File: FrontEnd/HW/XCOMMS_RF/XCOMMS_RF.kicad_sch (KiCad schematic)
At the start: 54 parts, among them J1 SMA, J2 SMA, J3 SFC-110-T2-F-D-A-TR, U1 SIM-14+, U2 HMC788ALP2ETR, U3 HMC952ALP5GE, U5 HMC788ALP2ETR, U6 AD8031, U7 ADT7310

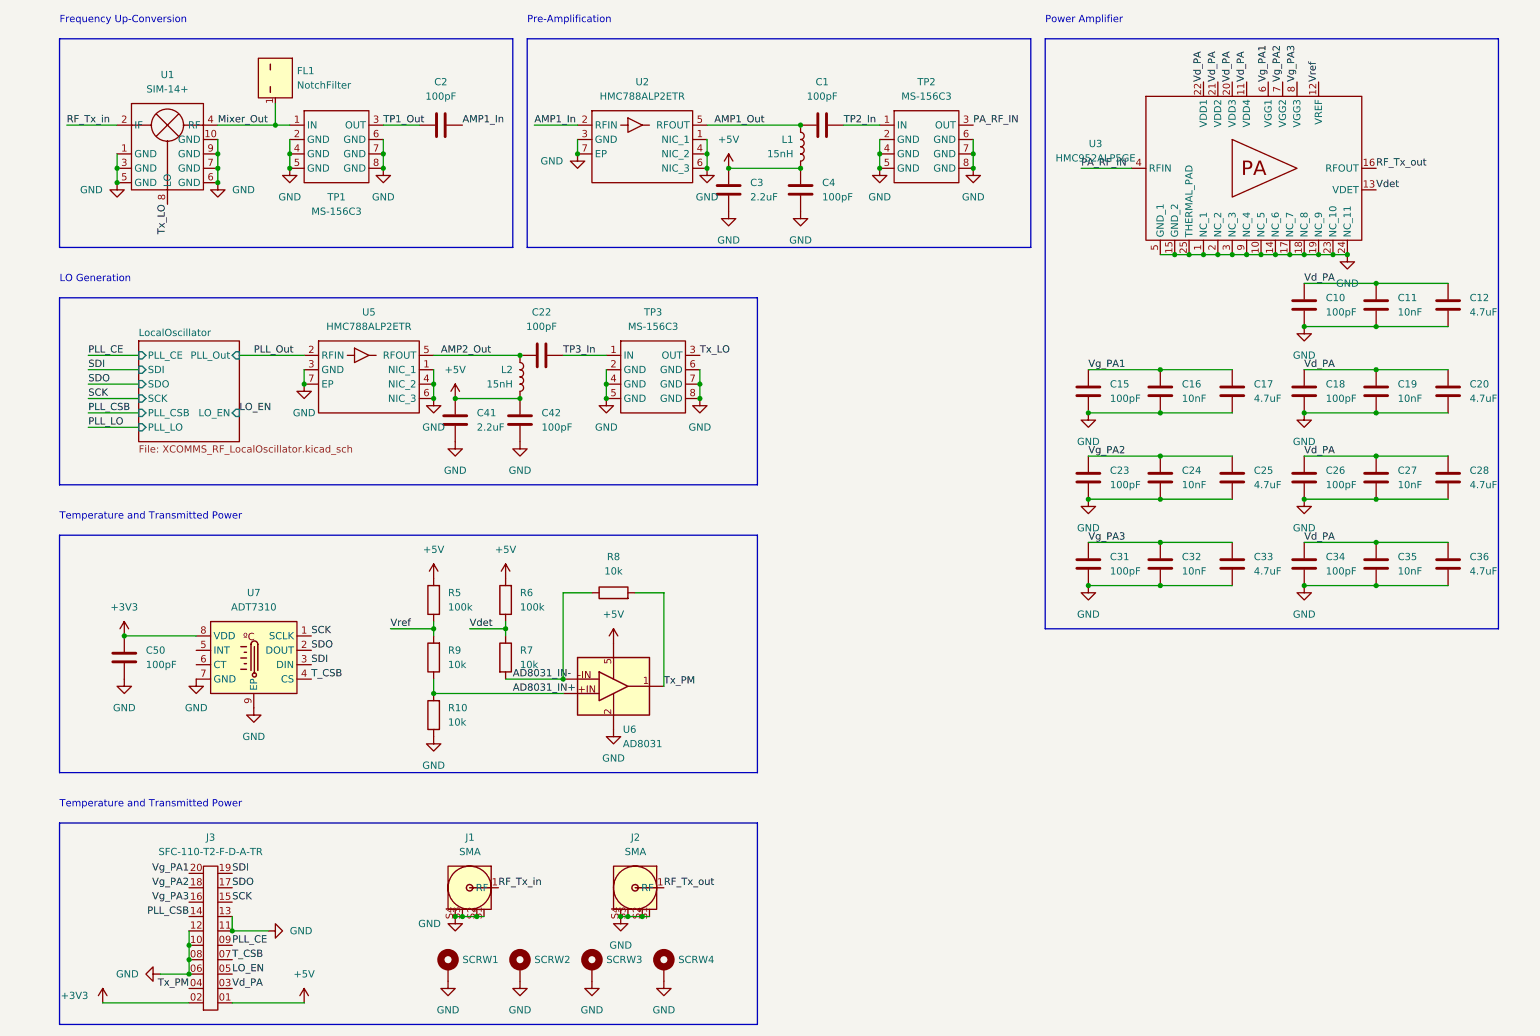
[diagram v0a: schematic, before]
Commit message: XCOMMS_RF update
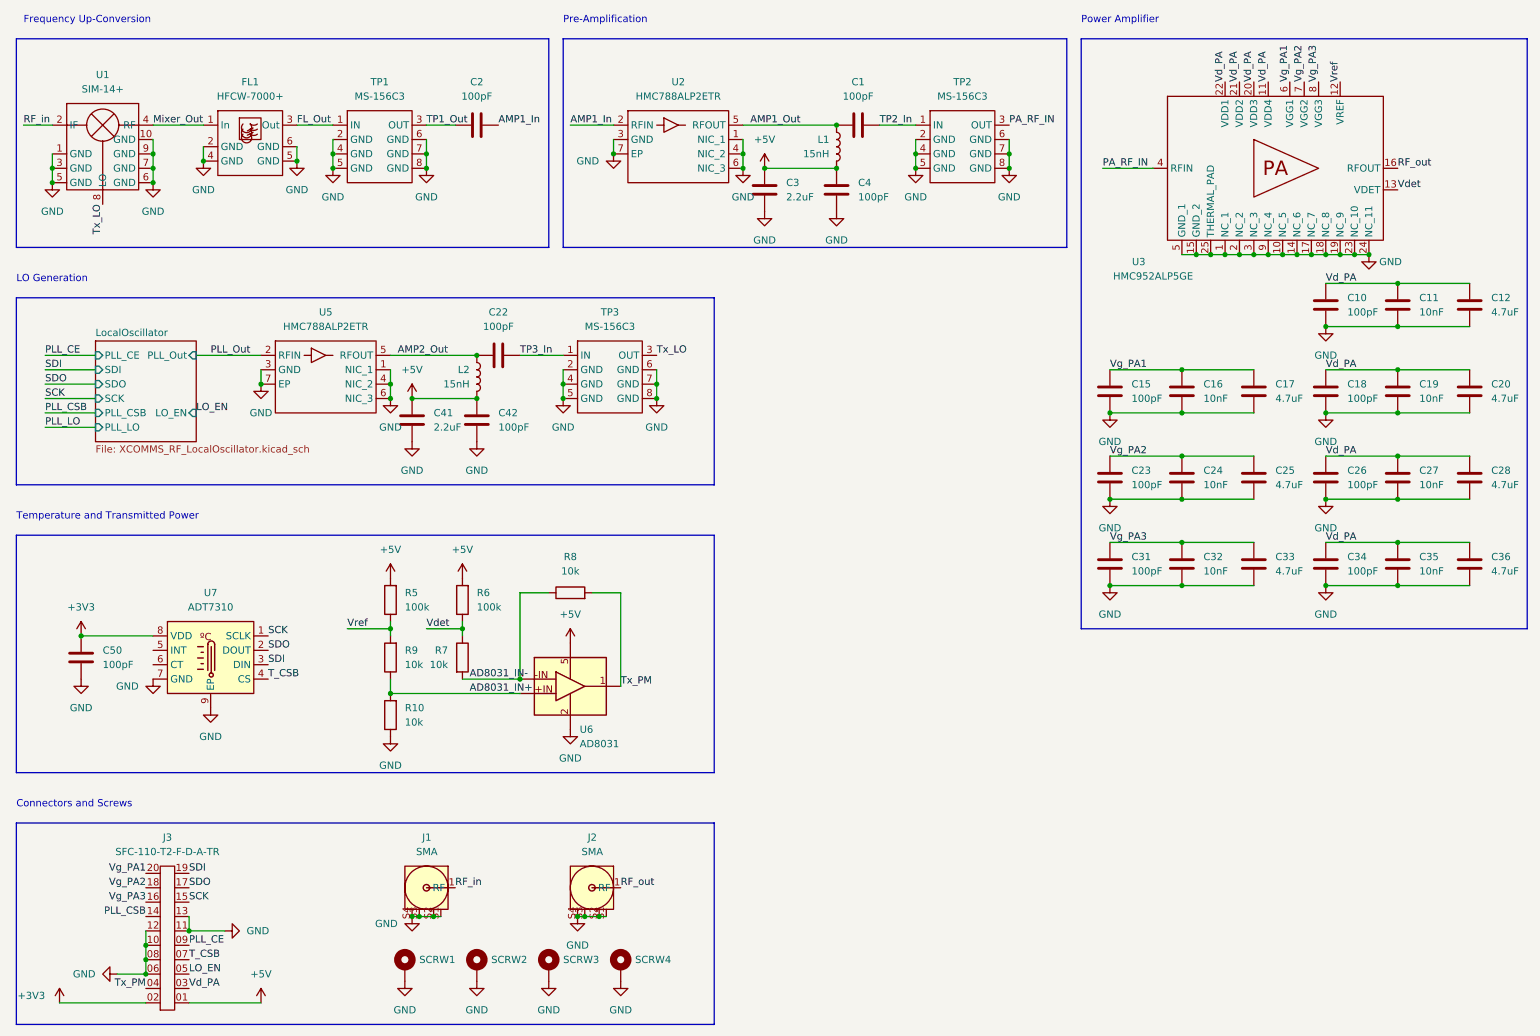
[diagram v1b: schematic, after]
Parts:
- removed FL1: NotchFilter, Notch_5600to6100MHz, symbol XCOMMS_RF-altium-import:1_NotchFilter
- added FL1: HFCW-7000+, GGS_RF:JC0603C, symbol GGS_RF:HFCW-7000+
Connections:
- net GND: now also FL1.2 (GND), FL1.4 (GND), FL1.5 (GND), FL1.6 (GND)
- net Mixer_Out: now also FL1.1 (In); no longer TP1.1 (IN)
- net RF_Tx_in renamed RF_in
- net RF_Tx_out renamed RF_out
- new net FL_Out: FL1.3 (Out), TP1.1 (IN)
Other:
- note added: "Connectors and Screws"
- moved on the sheet: C1, C10, C11, C12, C15, C16, C17, C18, C19, C2, C20, C22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

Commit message: PA TB
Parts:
- SCRW1: footprint MountingHole:MountingHole_3.2mm_M3_Pad_Via -> MountingHole:MountingHole_2.7mm_M2.5_Pad_Via
- SCRW2, SCRW3, SCRW4: footprint MountingHole:MountingHole_3.2mm_M3_Pad_Via -> MountingHole:MountingHole_2.7mm_Pad_Via
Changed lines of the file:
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@@
   (symbol (lib_id "power:GND") (at 21.59 45.72 0) (unit 1)
     (in_bom yes) (on_board yes) (fields_autoplaced)
-    (property "Reference" "#PWR?" (id 0) (at 21.59 52.07 0)
+    (property "Reference" "#PWR0109" (id 0) (at 21.59 52.07 0)
       (effects (font (size 1.27 1.27)) hide)
     )
@@
       (effects (font (size 1.27 1.27)) hide)
     )
-    (property "Footprint" "MountingHole:MountingHole_3.2mm_M3_Pad_Via" (id 2) (at 121.92 184.15 0)
+    (property "Footprint" "MountingHole:MountingHole_2.7mm_Pad_Via" (id 2) (at 121.92 184.15 0)
       (effects (font (size 1.27 1.27)) hide)
     )
@@
   (symbol (lib_id "power:GND") (at 64.77 41.91 0) (unit 1)
     (in_bom yes) (on_board yes) (fields_autoplaced)
-    (property "Reference" "#PWR?" (id 0) (at 64.77 48.26 0)
+    (property "Reference" "#PWR0175" (id 0) (at 64.77 48.26 0)
       (effects (font (size 1.27 1.27)) hide)
     )
@@
       (effects (font (size 1.27 1.27)) (justify left) hide)
     )
-    (property "Footprint" "MountingHole:MountingHole_3.2mm_M3_Pad_Via" (id 2) (at 109.22 184.15 0)
+    (property "Footprint" "MountingHole:MountingHole_2.7mm_Pad_Via" (id 2) (at 109.22 184.15 0)
       (effects (font (size 1.27 1.27)) hide)
     )
@@
       (effects (font (size 1.27 1.27)) hide)
     )
-    (property "Footprint" "MountingHole:MountingHole_3.2mm_M3_Pad_Via" (id 2) (at 96.52 184.15 0)
+    (property "Footprint" "MountingHole:MountingHole_2.7mm_Pad_Via" (id 2) (at 96.52 184.15 0)
       (effects (font (size 1.27 1.27)) hide)
     )
@@
       (effects (font (size 1.27 1.27)) (justify left) hide)
     )
-    (property "Footprint" "MountingHole:MountingHole_3.2mm_M3_Pad_Via" (id 2) (at 83.82 184.15 0)
+    (property "Footprint" "MountingHole:MountingHole_2.7mm_M2.5_Pad_Via" (id 2) (at 83.82 184.15 0)
       (effects (font (size 1.27 1.27)) hide)
     )
@@
   (symbol (lib_id "power:GND") (at 48.26 41.91 0) (unit 1)
     (in_bom yes) (on_board yes) (fields_autoplaced)
-    (property "Reference" "#PWR?" (id 0) (at 48.26 48.26 0)
+    (property "Reference" "#PWR0174" (id 0) (at 48.26 48.26 0)
       (effects (font (size 1.27 1.27)) hide)
     )
@@
   (symbol (lib_id "power:GND") (at 39.37 45.72 0) (unit 1)
     (in_bom yes) (on_board yes) (fields_autoplaced)
-    (property "Reference" "#PWR?" (id 0) (at 39.37 52.07 0)
+    (property "Reference" "#PWR0112" (id 0) (at 39.37 52.07 0)
       (effects (font (size 1.27 1.27)) hide)
     )
@@
       (reference "#PWR0108") (unit 1) (value "+5V") (footprint "")
     )
+    (path "/07bafb91-99e2-4082-8b6e-8175bdd2c01b"
+      (reference "#PWR0109") (unit 1) (value "GND") (footprint "")
+    )
     (path "/4040a07f-25cf-447d-98d2-351b395831b3"
       (reference "#PWR0110") (unit 1) (value "GND") (footprint "")
@@
       (reference "#PWR0111") (unit 1) (value "GND") (footprint "")
     )
+    (path "/a6692cd4-96b3-443d-8be6-accd4301b028"
+      (reference "#PWR0112") (unit 1) (value "GND") (footprint "")
+    )
     (path "/3bb43694-2f07-402c-9bac-c54bf6410d8e"
       (reference "#PWR0113") (unit 1) (value "GND") (footprint "")
@@
       (reference "#PWR0173") (unit 1) (value "GND") (footprint "")
     )
+    (path "/55f92a59-8c39-45cc-91eb-7b2e753eba53"
+      (reference "#PWR0174") (unit 1) (value "GND") (footprint "")
+    )
+    (path "/17fccb23-1284-49b1-b8e0-e599e0db79ac"
+      (reference "#PWR0175") (unit 1) (value "GND") (footprint "")
+    )
     (path "/6313534e-7526-48a8-a898-3b99488869c2"
       (reference "#PWR0177") (unit 1) (value "GND") (footprint "")
@@
       (reference "#PWR0187") (unit 1) (value "+5V") (footprint "")
     )
-    (path "/07bafb91-99e2-4082-8b6e-8175bdd2c01b"
-      (reference "#PWR?") (unit 1) (value "GND") (footprint "")
-    )
-    (path "/17fccb23-1284-49b1-b8e0-e599e0db79ac"
-      (reference "#PWR?") (unit 1) (value "GND") (footprint "")
-    )
-    (path "/55f92a59-8c39-45cc-91eb-7b2e753eba53"
-      (reference "#PWR?") (unit 1) (value "GND") (footprint "")
-    )
-    (path "/a6692cd4-96b3-443d-8be6-accd4301b028"
-      (reference "#PWR?") (unit 1) (value "GND") (footprint "")
-    )
     (path "/d3ecef9c-fb94-4e9d-927d-bb7dc8fea0fd"
       (reference "C1") (unit 1) (value "100pF") (footprint "Capacitor_SMD:C_0402_1005Metric")
@@
     )
     (path "/49ea3d04-dd55-4ffb-af0f-4dbf09c54d88"
-      (reference "SCRW1") (unit 1) (value "MountingHole_Pad") (footprint "MountingHole:MountingHole_3.2mm_M3_Pad_Via")
+      (reference "SCRW1") (unit 1) (value "MountingHole_Pad") (footprint "MountingHole:MountingHole_2.7mm_M2.5_Pad_Via")
     )
     (path "/2e497b62-365a-49a8-8171-e5b9c1dc77d6"
-      (reference "SCRW2") (unit 1) (value "MountingHole_Pad") (footprint "MountingHole:MountingHole_3.2mm_M3_Pad_Via")
+      (reference "SCRW2") (unit 1) (value "MountingHole_Pad") (footprint "MountingHole:MountingHole_2.7mm_Pad_Via")
     )
     (path "/227398ff-7060-4354-a52f-5d194ba6472b"
-      (reference "SCRW3") (unit 1) (value "MountingHole_Pad") (footprint "MountingHole:MountingHole_3.2mm_M3_Pad_Via")
+      (reference "SCRW3") (unit 1) (value "MountingHole_Pad") (footprint "MountingHole:MountingHole_2.7mm_Pad_Via")
     )
     (path "/0c48b150-3145-4990-a667-72f5d61838fc"
-      (reference "SCRW4") (unit 1) (value "MountingHole_Pad") (footprint "MountingHole:MountingHole_3.2mm_M3_Pad_Via")
+      (reference "SCRW4") (unit 1) (value "MountingHole_Pad") (footprint "MountingHole:MountingHole_2.7mm_Pad_Via")
     )
     (path "/d4ec1feb-fe93-44fc-98b1-414acb3250de"
